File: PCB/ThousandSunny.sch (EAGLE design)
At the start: 26 parts, among them IC1 LM317LZ

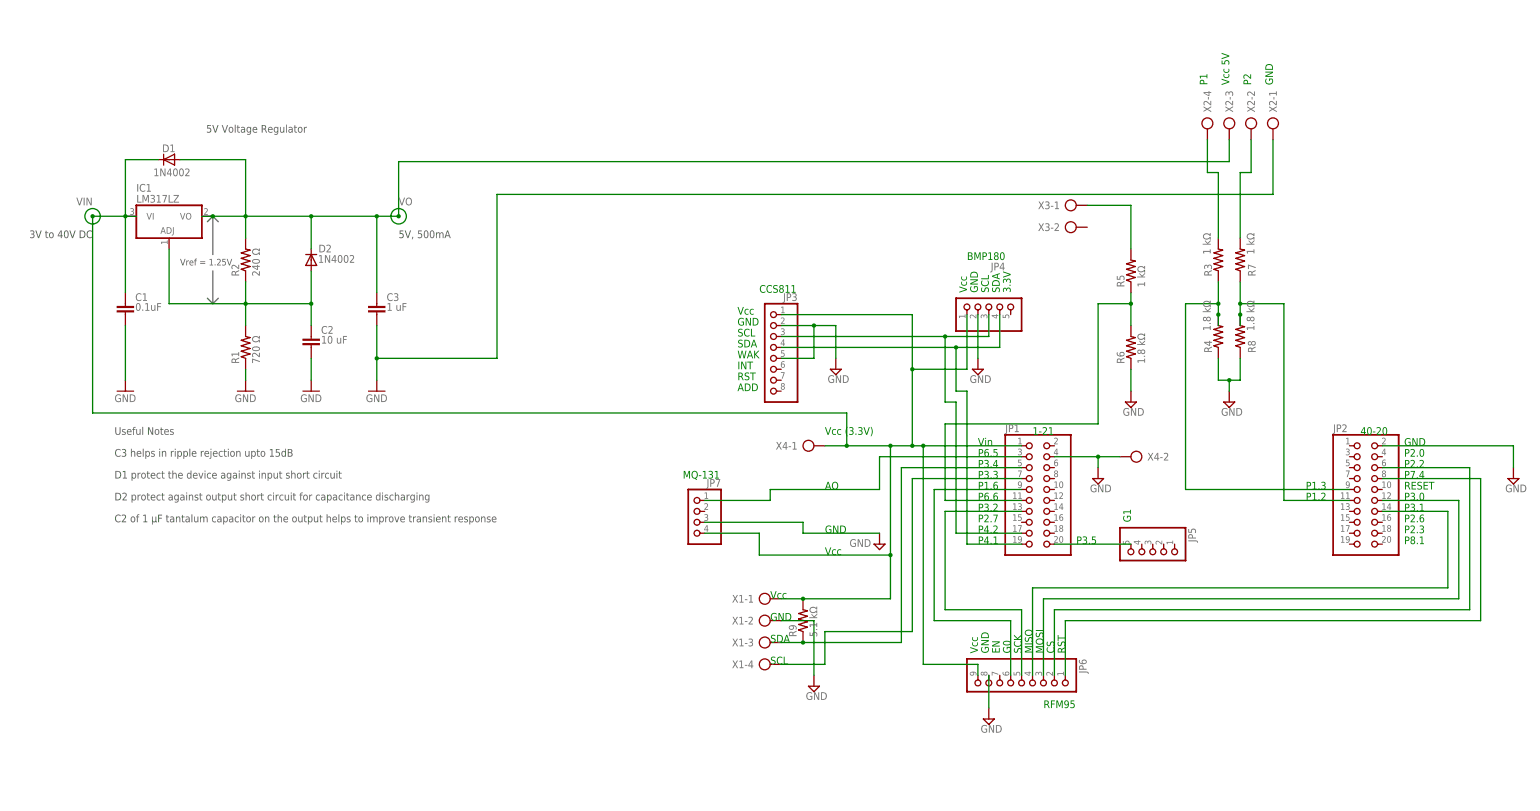
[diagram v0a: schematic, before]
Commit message: Board Bill of Materials
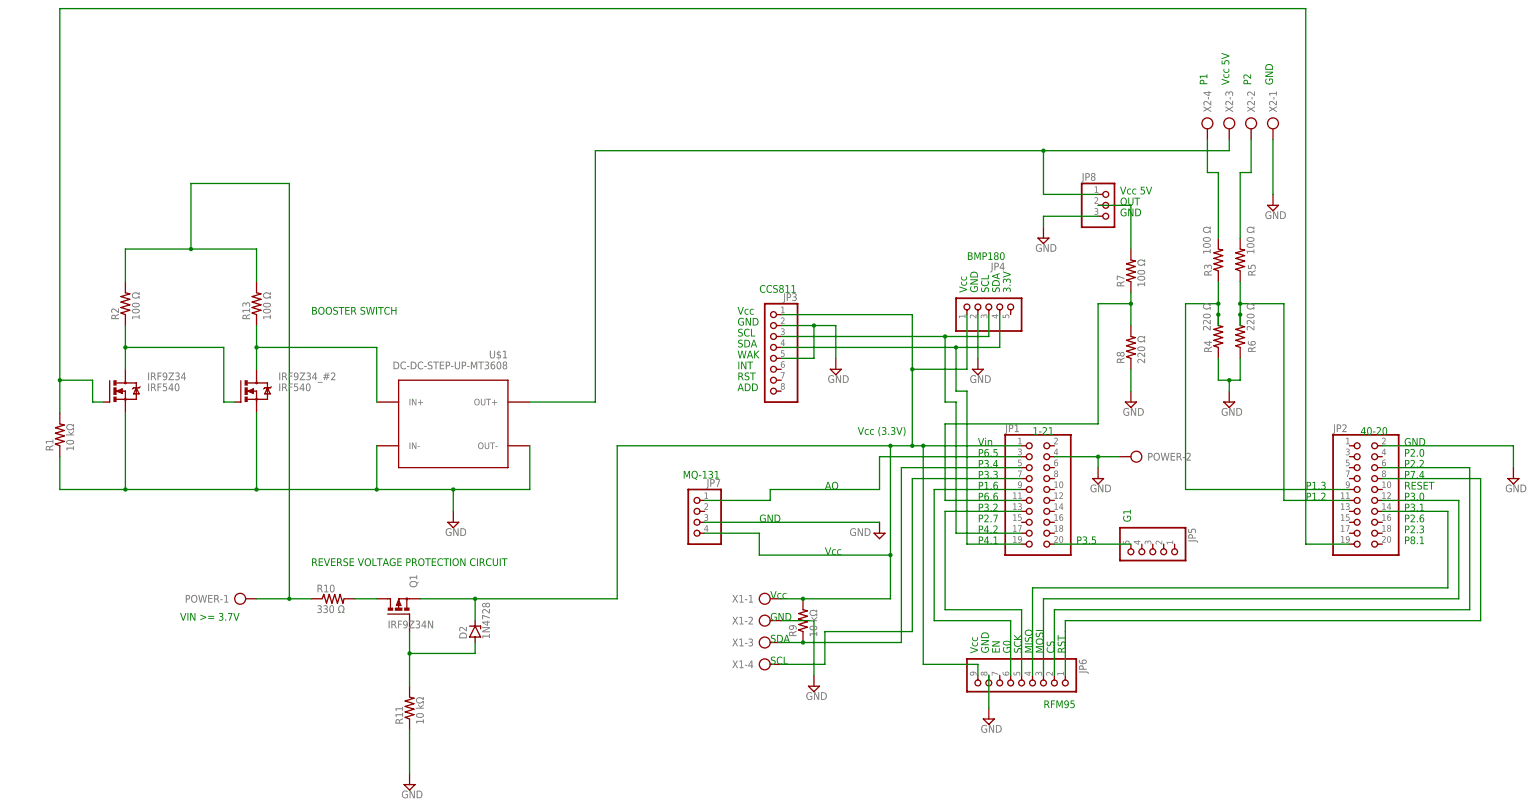
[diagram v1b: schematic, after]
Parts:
- removed C1: 0.1uF, rcl:C-EU075-052X106
- removed C2: 10 uF, rcl:C-EU075-052X106
- removed C3: 1 uF, rcl:C-EU075-052X106
- removed D1: 1N4002, diode:1N4004
- removed IC1: LM317LZ, linear:LM317LZ
- removed X3, X4: (no value), con-ptr500:AK300/2
- added IRF9Z34, IRF9Z34_#2: IRF540, transistor-power:IRF540
- added JP8: (no value), pinhead:PINHD-1X3
- added POWER: (no value), con-ptr500:AK300/2
- added Q1: IRF9Z34N, transistor-power:PMOSFET_PTO220BV
- added R10: 330 Ω, resistor:R-US_0204/7
- added R11: 10 kΩ, resistor:R-US_0204/7
- added R13: 100 Ω, resistor:R-US_0204/7
- added U$1: DC-DC-STEP-UP-MT3608, dc-dc-boost-2a-microusb-mt3608:DC-DC-STEP-UP-MT3608
- D2: value 1N4002 -> 1N4728; device diode:1N4004 -> diode:1N4728
- R1: value 720 Ω -> 10 kΩ; device rcl:R-US_0204/5 -> resistor:R-US_0204/7
- R2: value 240 Ω -> 100 Ω; device rcl:R-US_0204/5 -> resistor:R-US_0204/7
- R3, R5, R7: value 1 kΩ -> 100 Ω; device rcl:R-US_0204/5 -> resistor:R-US_0204/7
- R4, R6, R8: value 1.8 kΩ -> 220 Ω; device rcl:R-US_0204/5 -> resistor:R-US_0204/7
- R9: value 5.1 kΩ -> 10 kΩ; device rcl:R-US_0204/5 -> resistor:R-US_0204/7
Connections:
- net N$15 renamed RAW_P1
- net P1.3 renamed DUST_P1
- net P1.6 renamed RFM95W_G0
- net P2.2 renamed RFM95W_CS
- net P3.0 renamed MOSI
- net P3.1 renamed MISO
- net P3.2 renamed SCK
- net P3.3 renamed SHT_CLOCK
- net P3.4 renamed SHT_DATA
- net P3.5 renamed G1
- net P4.1 renamed SDA
- net P4.2 renamed SCL
- net P6.5 renamed O3
- net P7.4 renamed RFM95_RST
- removed net N$17: R7.2, X2-2.KL
- removed net N$18: R5.2, X3-1.KL
- removed net N$2: C2.1, D2.A, IC1.ADJ, R1.2, R2.1
- removed net P1.2: JP2.11, R7.1, R8.2
- removed net P6.6: JP1.11, R5.1, R6.2
- removed net VIN: C1.1, D1.C, IC1.VI, JP1.1, JP3.1, JP4.1, JP6.9, JP7.4, R9.2, X1-1.KL, X4-1.KL
- removed net VO: C3.1, D1.A, D2.C, IC1.VO, R2.2, X2-3.KL
- new net ANODE: D2.A, Q1.G, R11.2
- new net BATTERY: POWER-1.KL, R10.1, R13.2, R2.2
- new net D1->G2: IRF9Z34.D, IRF9Z34_#2.G, R2.1
- new net D2->VIN: IRF9Z34_#2.D, R13.1, U$1.IN+
- new net DRAIN_Q1: Q1.D, R10.2
- new net DUST_P2: JP2.11, R5.1, R6.2
- new net P8.2: IRF9Z34.G, JP2.19, R1.2
- new net RAW_P2: R5.2, X2-2.KL
- new net RAW_SOLAR: JP8.2, R7.2
- new net SOLAR: JP1.11, R7.1, R8.2
- new net VIN->DUST: JP8.1, U$1.OUT+, X2-3.KL
- new net VZ->3.3V: D2.C, JP1.1, JP3.1, JP4.1, JP6.9, JP7.4, Q1.S, R9.2, X1-1.KL
- net GND: now also IRF9Z34.S, IRF9Z34_#2.S, JP8.3, POWER-2.KL, R11.1, U$1.IN-, U$1.OUT-; no longer C1.2, C2.2, C3.2, X4-2.KL
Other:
- note added: "BOOSTER SWITCH"
- note added: "OUT"
- note added: "REVERSE VOLTAGE PROTECTION CIRCUIT"
- note added: "VIN >= 3.7V"
- note removed: "3V to 40V DC"
- note removed: "5V Voltage Regulator"
- note removed: "5V, 500mA"
- note removed: "C2 of 1 µF tantalum capacitor on the output helps to improve transient response"
- note removed: "C3 helps in ripple rejection upto 15dB"
- note removed: "D1 protect the device against input short circuit"
- note removed: "D2 protect against output short circuit for capacitance discharging"
- note removed: "Useful Notes"
- note removed: "Vref = 1.25V"
- moved on the sheet: R1, R2, R5, R6, R7, R8
